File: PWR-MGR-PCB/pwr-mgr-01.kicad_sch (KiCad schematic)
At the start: 26 parts, among them J3 USB_C_Receptacle_USB2.0_14P, U1 BQ24075, U5 USBLC6-2SC6, U6 TPS631011YBGR-Pin_Corrected

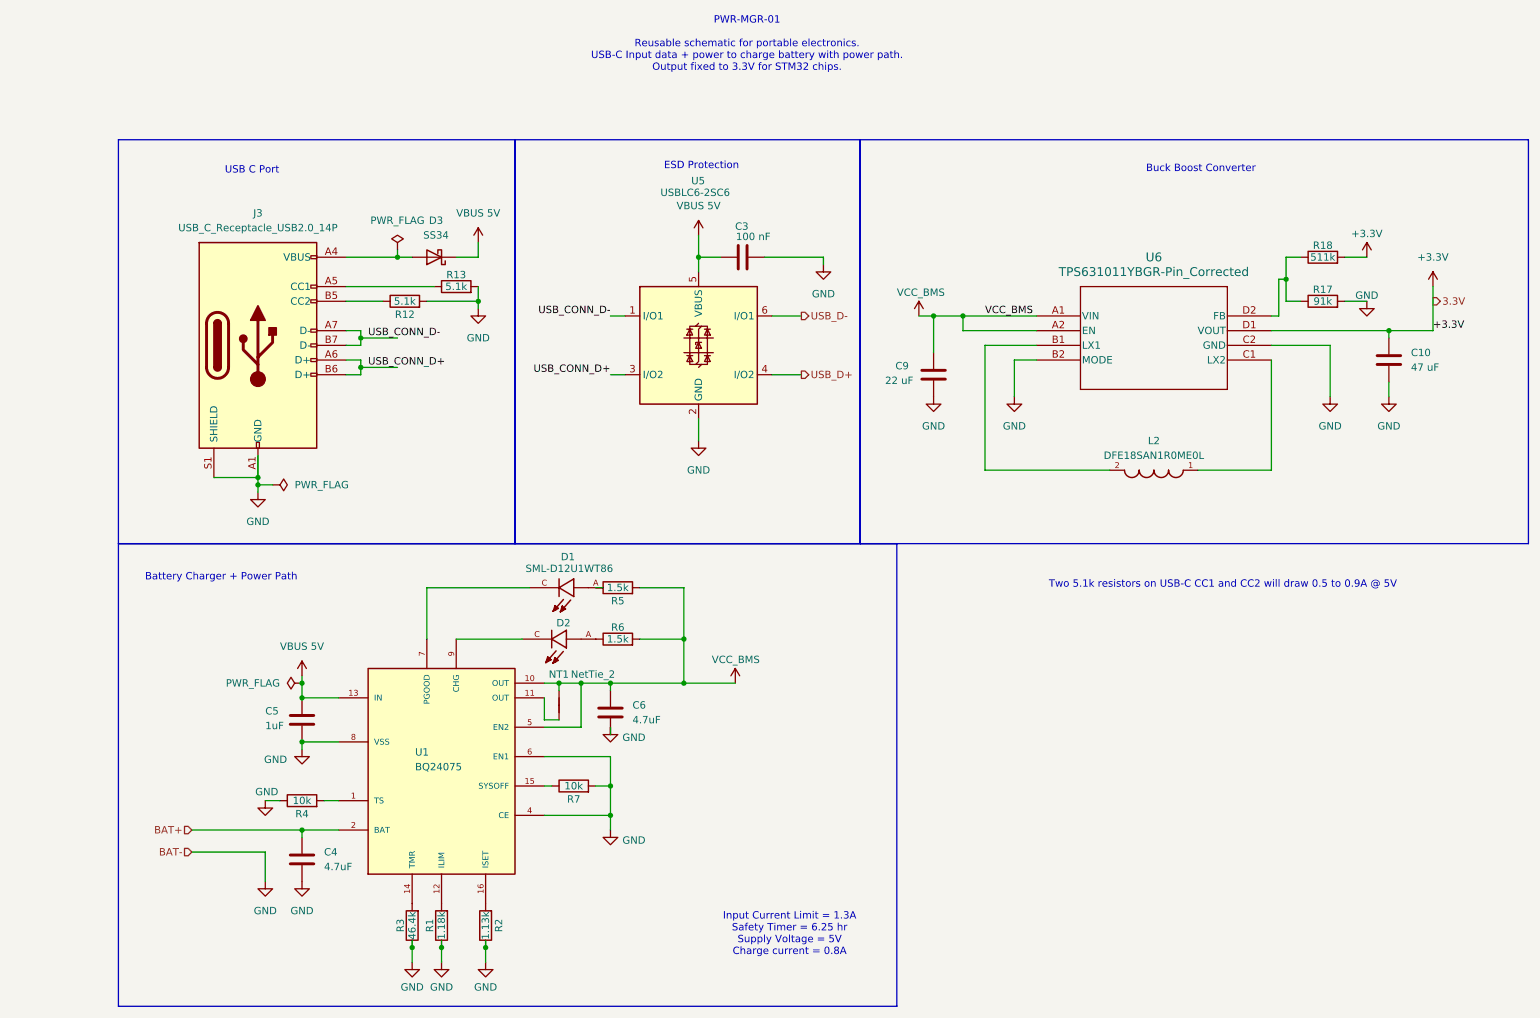
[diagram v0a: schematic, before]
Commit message: begin v2, update schematic
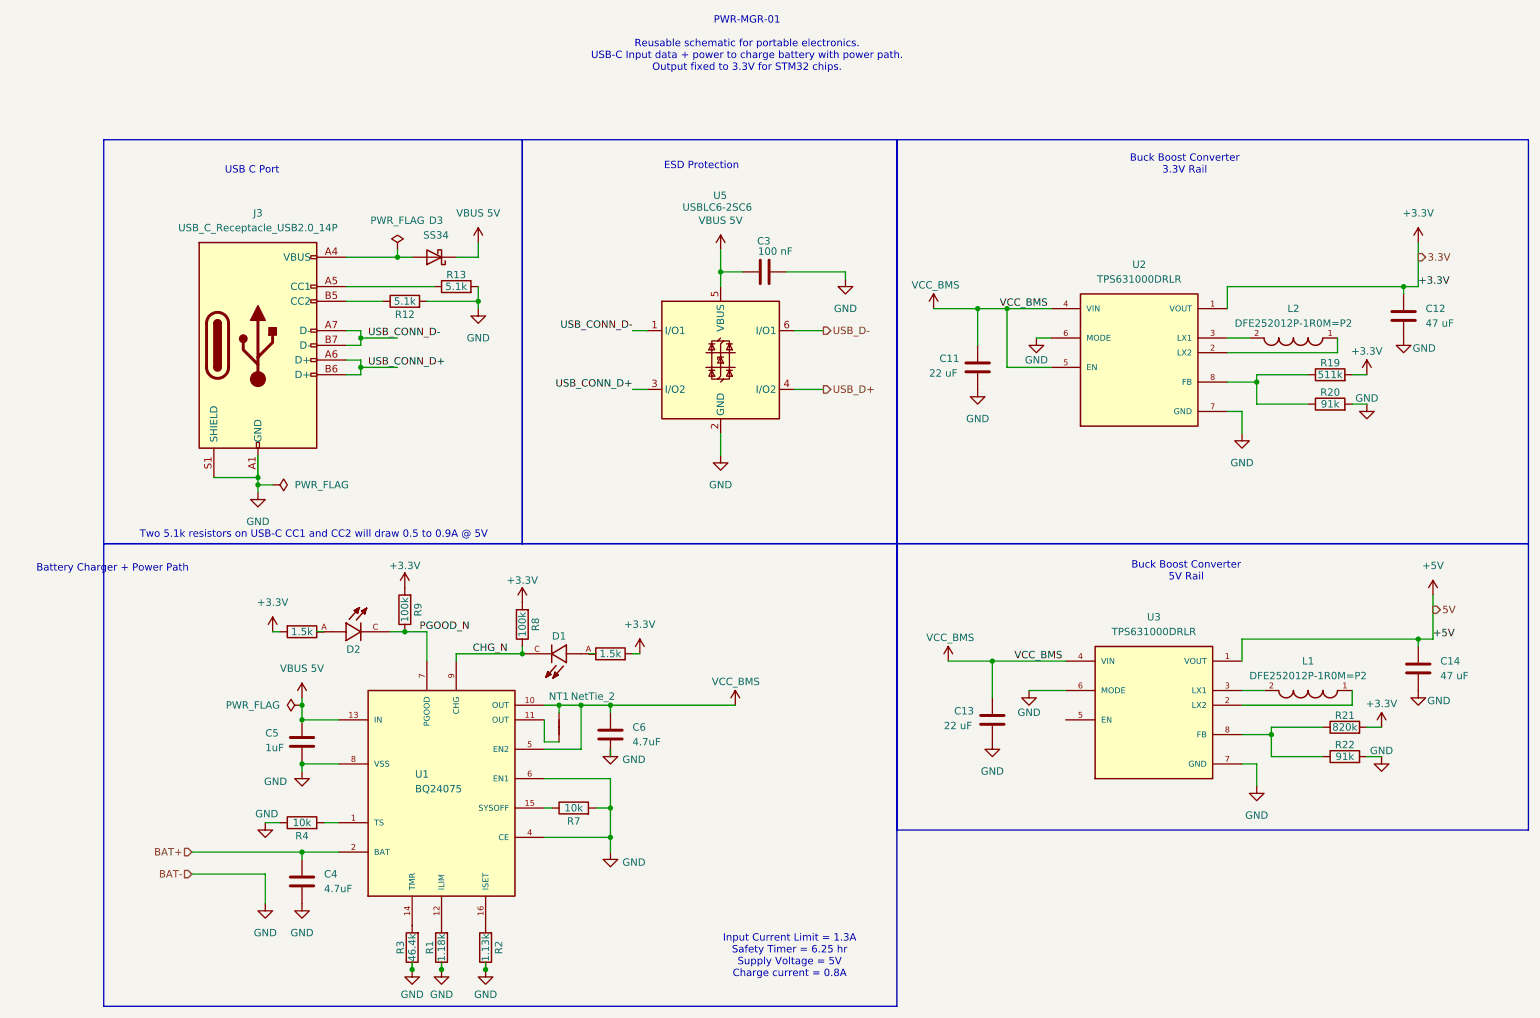
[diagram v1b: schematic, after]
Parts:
- removed C10: 47 uF, Capacitor_SMD:C_0805_2012Metric, symbol Device:C
- removed C9: 22 uF, Capacitor_SMD:C_0805_2012Metric, symbol Device:C
- removed L2: DFE18SAN1R0ME0L, DFE18SAN1ROMEO Inductor:INDC1608X80N, symbol DFE18SAN1R0ME0L:DFE18SAN1R0ME0L
- removed R17: 91k, Resistor_SMD:R_0805_2012Metric, symbol Device:R
- removed R18: 511k, Resistor_SMD:R_0805_2012Metric, symbol Device:R
- removed U6: TPS631011YBGR-Pin_Corrected, DSBGA8_YBG_TEX, symbol TPS631011:TPS631011YBGR-Pin_Corrected
- added C11, C13: 22 uF, Capacitor_SMD:C_0805_2012Metric, symbol Device:C
- added C12, C14: 47 uF, Capacitor_SMD:C_0805_2012Metric, symbol Device:C
- added L1, L2: DFE252012P-1R0M=P2, DFE252012P-1R0M=P2:INDC2520X120N, symbol DFE252012P-1R0M_P2:DFE252012P-1R0M=P2
- added R19: 511k, Resistor_SMD:R_0805_2012Metric, symbol Device:R
- added R20, R22: 91k, Resistor_SMD:R_0805_2012Metric, symbol Device:R
- added R21: 820k, Resistor_SMD:R_0805_2012Metric, symbol Device:R
- added R8, R9: 100k, Resistor_SMD:R_0805_2012Metric, symbol Device:R
- added U2, U3: TPS631000DRLR, TPS631000DRLR:SOT50P160X60-8N, symbol TPS631000DRLR:TPS631000DRLR
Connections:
- net +3.3V: now also R5.2, R6.2, C12.1, R19.2, R21.2, R8.2, R9.2, U2.1 (VOUT)
- net GND: now also C11.2, C12.2, C13.2, C14.2, R20.2, R22.2, U2.6 (MODE), U2.7 (GND), U3.6 (MODE), U3.7 (GND)
- net VCC_BMS: now also C11.1, C13.1, U2.4 (VIN), U2.5 (EN), U3.4 (VIN); no longer R5.2, R6.2
- net CHG_N: now reaches D1.C
- net CHG_N: now also U1.9 (CHG), R8.1; no longer U1.7 (PGOOD)
- net PGOOD_N: now reaches D2.C
- net PGOOD_N: now also U1.7 (PGOOD), R9.1; no longer U1.9 (CHG)
- new net: R19.1, R20.1, U2.8 (FB)
- new net: L2.1, U2.2 (LX2)
- new net: L2.2, U2.3 (LX1)
- new net: L1.1, U3.2 (LX2)
- new net: L1.2, U3.3 (LX1)
- new net: R21.1, R22.1, U3.8 (FB)
- new net +5V: C14.1, U3.1 (VOUT)
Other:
- note added: "Buck Boost Converter 3.3V Rail"
- note added: "Buck Boost Converter 5V Rail"
- note removed: "Buck Boost Converter"
- moved on the sheet: C3, C4, C5, C6, D1, NT1, R1, R2, R3, R4, R7, U1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
